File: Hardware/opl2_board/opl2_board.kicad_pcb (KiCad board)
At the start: 2 copper layers, 80.8 x 60.1 mm, 21 parts, among them J1 Conn_01x40, J2 AudioJack3, U1 74HC00, U2 YM3812, U3 YM3014B, U4 LM358, X1 3.579545 MHz

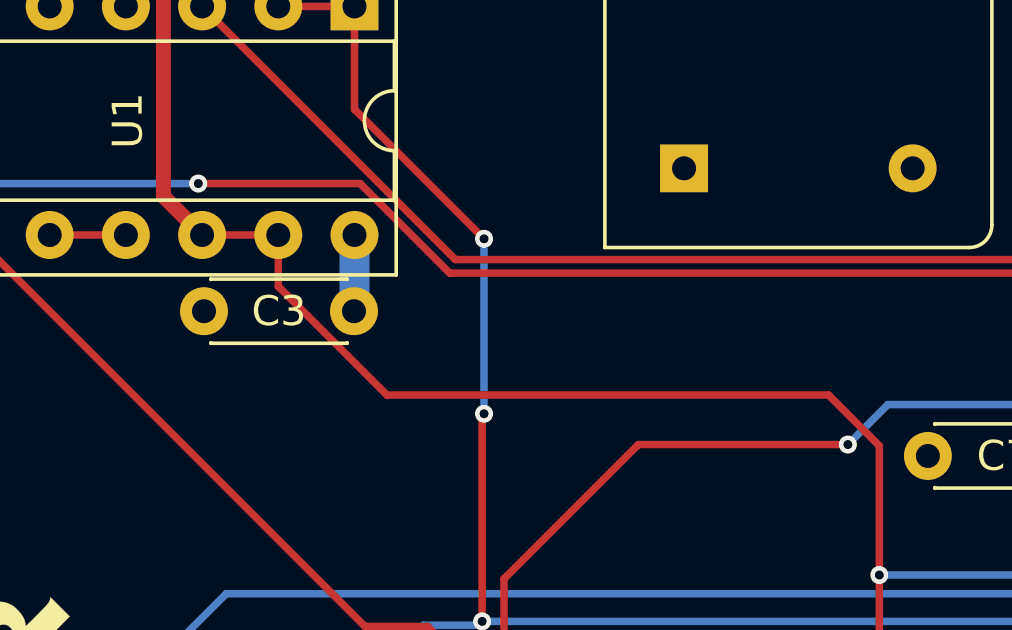
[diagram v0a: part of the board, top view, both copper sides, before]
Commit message: don't remember what I did there and diffs are useless :/
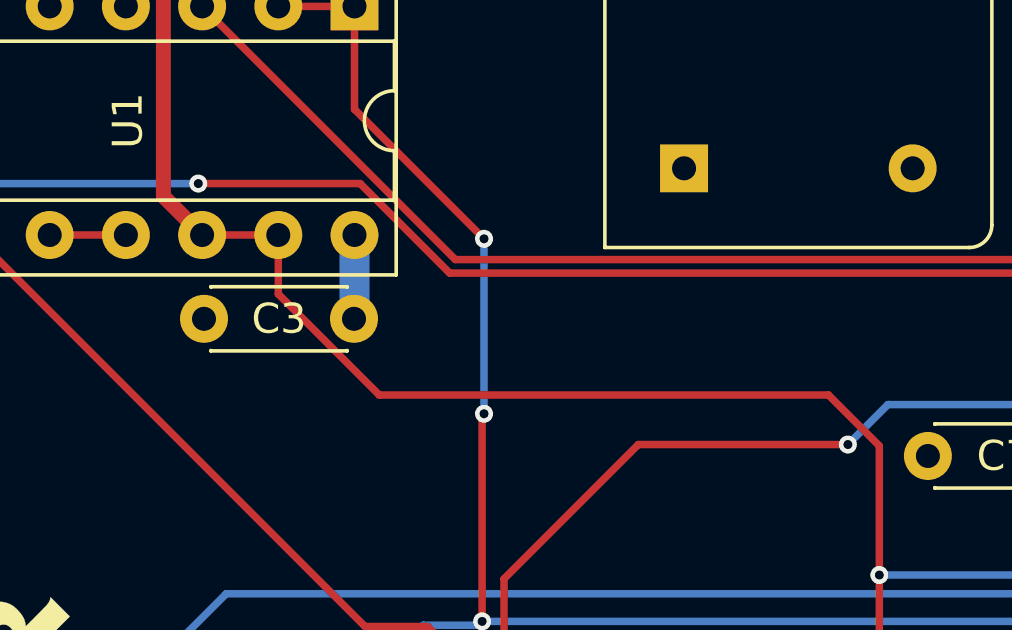
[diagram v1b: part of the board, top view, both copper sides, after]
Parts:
- moved C3 0.25 mm to (18.8, -18.0)
